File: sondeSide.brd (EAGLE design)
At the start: 105.2 x 31.8 mm, 41 parts

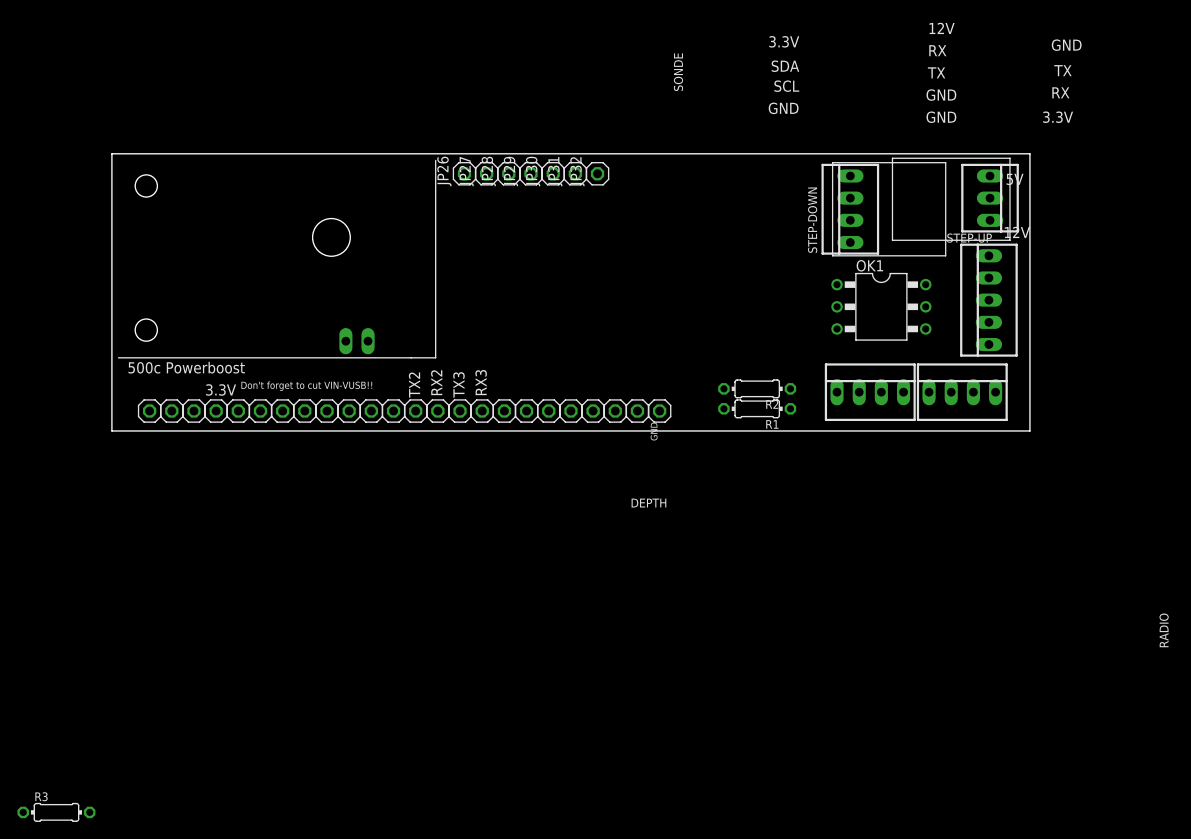
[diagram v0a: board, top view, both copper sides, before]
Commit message: About to do significant rerouting
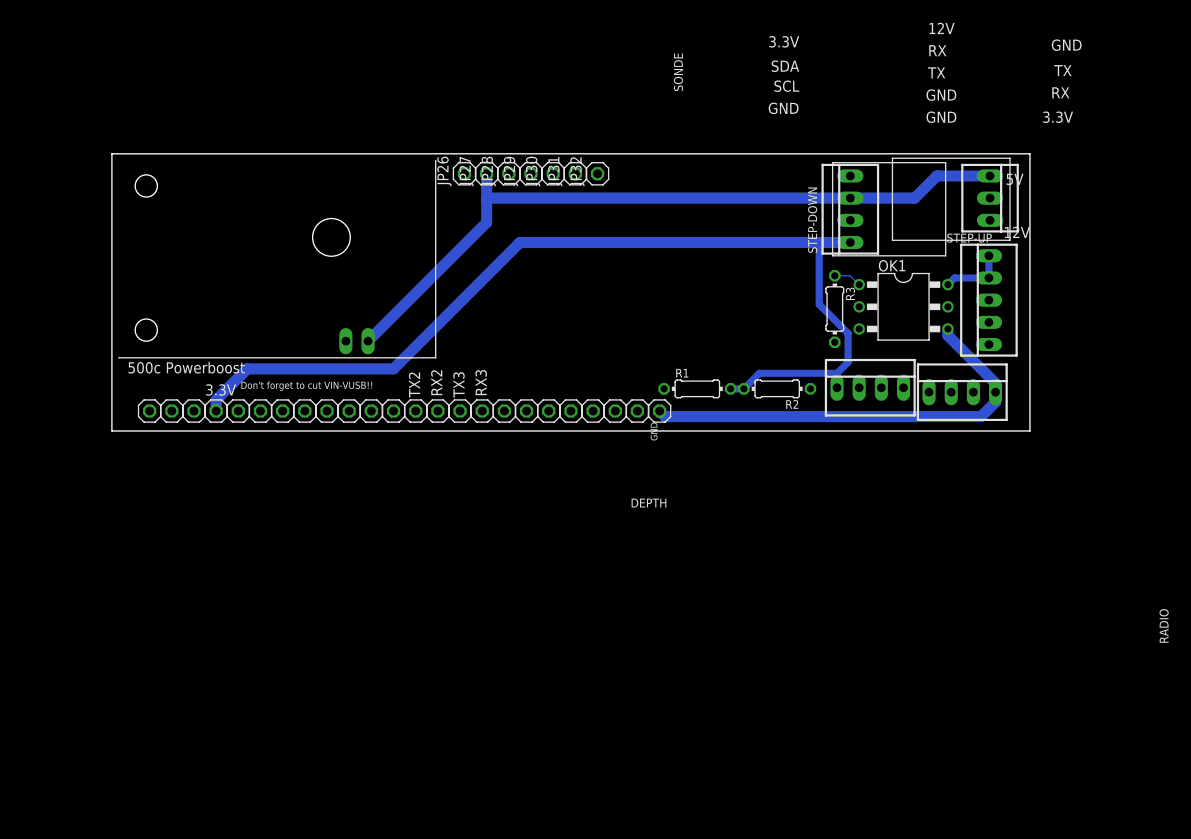
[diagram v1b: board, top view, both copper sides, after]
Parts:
- moved R3 106.2 mm to (82.8, 14.0), turned to 270 degrees
- moved R1 7.23 mm to (67.1, 4.83), turned to 0 degrees
- moved OK1 2.54 mm to (90.7, 14.2)
- moved R2 2.29 mm to (76.2, 4.83)
- moved RADIO 0.51 mm to (86.9, 4.95)
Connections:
- net GND: no longer PWRBOOST.1
- net GND_PLANE: now also PWRBOOST.1
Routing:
- net 3.3V: track 0.00 -> 116.4 mm
- net 5V: track 0.00 -> 83.6 mm
- net GND: track 0.00 -> 57.6 mm
- net N$1: track 0.00 -> 3.21 mm
